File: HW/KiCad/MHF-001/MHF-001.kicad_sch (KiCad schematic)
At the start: 199 parts, among them J1 DE15_Socket_HighDensity_Mount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, J2 Mini-DIN-6, J3 Conn_Coaxial, J4 Conn_02x32_Odd_Even, J5 USB_B_Micro, J6 Conn_02x32_Odd_Even, J8 AVR-ISP-6, M3 CY7C109D-10ZXI, M5 CY7C109D-10ZXI, Q1 BC107, U1 ATMEGA2560-16AU, U10 74HC245, U11 74HC245, U12 74HC245, U13 CH340G, U14 AMS1117-5.0, U15 AMS1117-3.3, U2 74HC14, U3 74LS08, U4 74HC165, U6 74AHC373PW, U7 74HC595, U8 74HC595, U9 74HC157, Y1 16 MHz, Y2 12 MHz

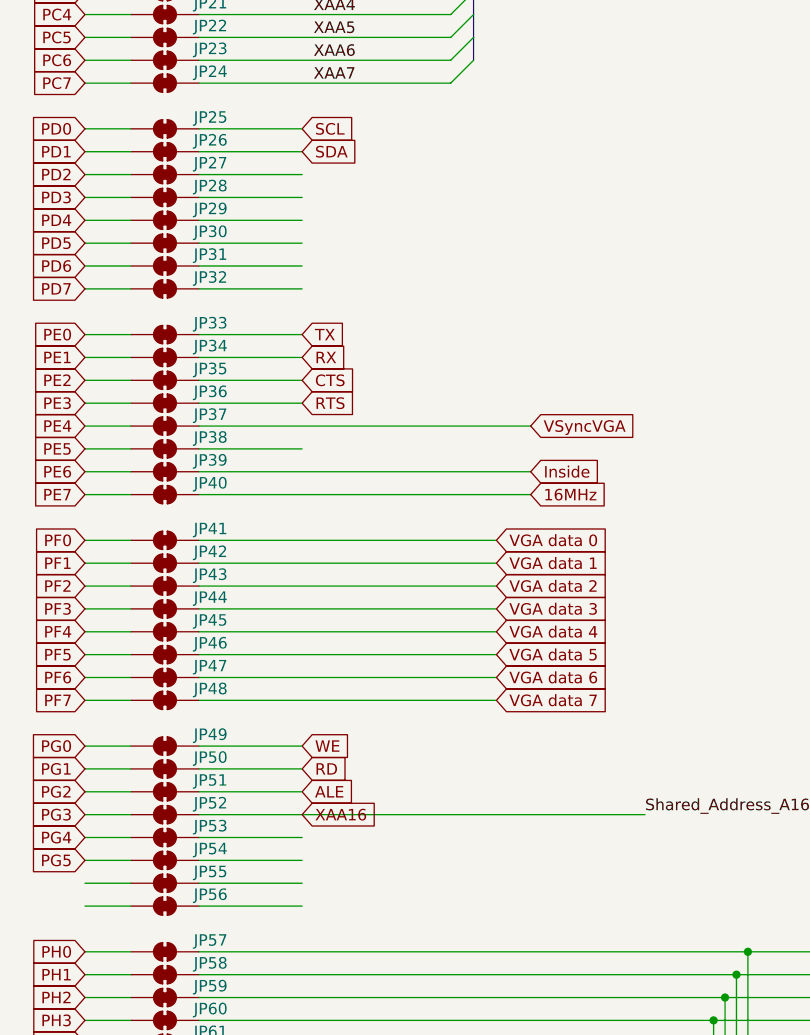
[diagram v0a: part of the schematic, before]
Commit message: some labels
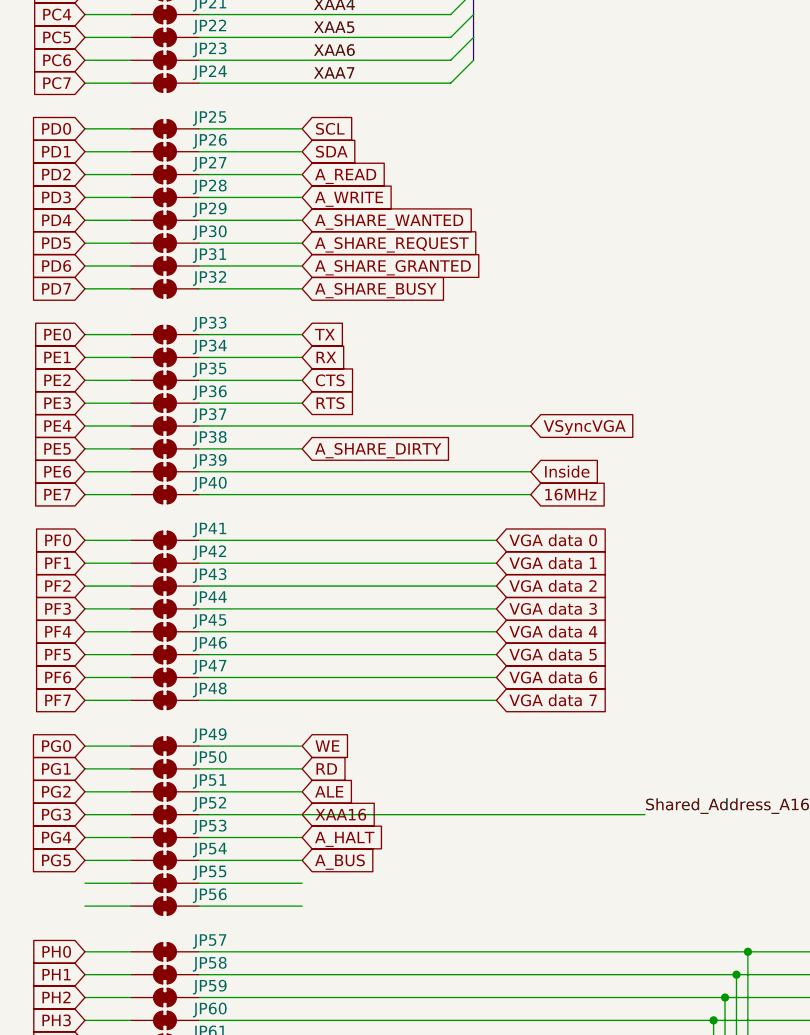
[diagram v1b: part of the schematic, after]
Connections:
- net A_BUS: now also JP54.2 (B)
- net A_HALT: now also JP53.2 (B)
- net A_READ: now also JP27.2 (B)
- net A_SHARE_BUSY: now also JP32.2 (B)
- net A_SHARE_DIRTY: now also JP38.2 (B)
- net A_SHARE_GRANTED: now also JP31.2 (B)
- net A_SHARE_REQUEST: now also JP30.2 (B)
- net A_SHARE_WANTED: now also JP29.2 (B)
- net A_WRITE: now also JP28.2 (B)
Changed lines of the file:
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@@
 		)
 	)
+	(global_label "A_SHARE_WANTED"
+		(shape input)
+		(at 675.64 426.72 0)
+		(fields_autoplaced yes)
+		(effects
+			(font
+				(size 1.27 1.27)
+			)
+			(justify left)
+		)
+		(property "Intersheetrefs" "${INTERSHEET_REFS}"
+			(at 694.9537 426.72 0)
+			(effects
+				(font
+					(size 1.27 1.27)
+				)
+				(justify left)
+				(hide yes)
+			)
+		)
+	)
 	(global_label "A[0..15]"
 		(shape input)
@@
 		)
 	)
+	(global_label "A_SHARE_REQUEST"
+		(shape input)
+		(at 675.64 429.26 0)
+		(fields_autoplaced yes)
+		(effects
+			(font
+				(size 1.27 1.27)
+			)
+			(justify left)
+		)
+		(property "Intersheetrefs" "${INTERSHEET_REFS}"
+			(at 696.1027 429.26 0)
+			(effects
+				(font
+					(size 1.27 1.27)
+				)
+				(justify left)
+				(hide yes)
+			)
+		)
+	)
 	(global_label "HSyncVGA"
 		(shape input)
@@
 		)
 	)
+	(global_label "A_SHARE_GRANTED"
+		(shape input)
+		(at 675.64 431.8 0)
+		(fields_autoplaced yes)
+		(effects
+			(font
+				(size 1.27 1.27)
+			)
+			(justify left)
+		)
+		(property "Intersheetrefs" "${INTERSHEET_REFS}"
+			(at 696.0423 431.8 0)
+			(effects
+				(font
+					(size 1.27 1.27)
+				)
+				(justify left)
+				(hide yes)
+			)
+		)
+	)
 	(global_label "PH1"
 		(shape input)
@@
 		)
 	)
+	(global_label "A_SHARE_DIRTY"
+		(shape input)
+		(at 675.64 452.12 0)
+		(fields_autoplaced yes)
+		(effects
+			(font
+				(size 1.27 1.27)
+			)
+			(justify left)
+		)
+		(property "Intersheetrefs" "${INTERSHEET_REFS}"
+			(at 692.8976 452.12 0)
+			(effects
+				(font
+					(size 1.27 1.27)
+				)
+				(justify left)
+				(hide yes)
+			)
+		)
+	)
 	(global_label "VGA data 5"
 		(shape input)
@@
 		)
 	)
+	(global_label "A_HALT"
+		(shape input)
+		(at 675.64 495.3 0)
+		(fields_autoplaced yes)
+		(effects
+			(font
+				(size 1.27 1.27)
+			)
+			(justify left)
+		)
+		(property "Intersheetrefs" "${INTERSHEET_REFS}"
+			(at 685.0962 495.3 0)
+			(effects
+				(font
+					(size 1.27 1.27)
+				)
+				(justify left)
+				(hide yes)
+			)
+		)
+	)
 	(global_label "Rf"
 		(shape input)
@@
 		)
 	)
+	(global_label "A_READ"
+		(shape input)
+		(at 675.64 421.64 0)
+		(fields_autoplaced yes)
+		(effects
+			(font
+				(size 1.27 1.27)
+			)
+			(justify left)
+		)
+		(property "Intersheetrefs" "${INTERSHEET_REFS}"
+			(at 685.459 421.64 0)
+			(effects
+				(font
+					(size 1.27 1.27)
+				)
+				(justify left)
+				(hide yes)
+			)
+		)
+	)
 	(global_label "A[0..15]"
 		(shape input)
@@
 		)
 	)
+	(global_label "A_SHARE_BUSY"
+		(shape input)
+		(at 675.64 434.34 0)
+		(fields_autoplaced yes)
+		(effects
+			(font
+				(size 1.27 1.27)
+			)
+			(justify left)
+		)
+		(property "Intersheetrefs" "${INTERSHEET_REFS}"
+			(at 692.5952 434.34 0)
+			(effects
+				(font
+					(size 1.27 1.27)
+				)
+				(justify left)
+				(hide yes)
+			)
+		)
+	)
 	(global_label "{RW,CLOCK,halt}"
 		(shape input)
@@
 		)
 	)
+	(global_label "A_WRITE"
+		(shape input)
+		(at 675.64 424.18 0)
+		(fields_autoplaced yes)
+		(effects
+			(font
+				(size 1.27 1.27)
+			)
+			(justify left)
+		)
+		(property "Intersheetrefs" "${INTERSHEET_REFS}"
+			(at 686.1242 424.18 0)
+			(effects
+				(font
+					(size 1.27 1.27)
+				)
+				(justify left)
+				(hide yes)
+			)
+		)
+	)
 	(global_label "SS"
 		(shape input)
@@
 				(hide yes)
 			)
+		)
+	)
+	(global_label "A_BUS"
+		(shape input)
+		(at 675.64 497.84 0)
+		(fields_autoplaced yes)
+		(effects
+			(font
+				(size 1.27 1.27)
+			)
+			(justify left)
+		)
+		(property "Intersheetrefs" "${INTERSHEET_REFS}"
+			(at 684.4914 497.84 0)
+			(effects
+				(font
+					(size 1.27 1.27)
+				)
+				(justify left)
+				(hide yes)
+			)

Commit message: schema MHF-001 maybe OK
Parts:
- removed sys_Addr1, sys_Addr2, sys_Data1: Conn_01x08, Connector_PinHeader_2.54mm:PinHeader_1x08_P2.54mm_Vertical, symbol Connector_Generic:Conn_01x08
- added J10: I2C, Connector_PinHeader_2.54mm:PinHeader_1x04_P2.54mm_Vertical, symbol Connector_Generic:Conn_01x04
- added J11: POWER, Connector_PinHeader_2.54mm:PinHeader_2x03_P2.54mm_Vertical, symbol Connector_Generic:Conn_02x03_Odd_Even
- added J7: SPI, Connector_PinHeader_2.54mm:PinHeader_1x06_P2.54mm_Vertical, symbol Connector_Generic:Conn_01x06
- added J9: Serial, Connector_PinHeader_2.54mm:PinHeader_1x06_P2.54mm_Vertical, symbol Connector_Generic:Conn_01x06
- added JP100, JP101, JP102, JP103, JP104, JP105, JP106, JP107, JP108, JP92, JP93, JP94, JP95, JP96, JP97, JP98, JP99: SolderJumper_3_Open, Jumper:SolderJumper-3_P1.3mm_Open_RoundedPad1.0x1.5mm, symbol Jumper:SolderJumper_3_Open
- added LED5, LED6: LED, LED_SMD:LED_0805_2012Metric, symbol Device:LED
- C10, C12, C13, C14, C15, C16, C2, C3, C4, C5, C6, C7, C8, C9: footprint Capacitor_SMD:C_0603_1608Metric -> Capacitor_SMD:C_0603_1608Metric_Pad1.08x0.95mm_HandSolder
- C11: footprint Capacitor_SMD:C_1206_3216Metric -> Capacitor_SMD:C_0603_1608Metric_Pad1.08x0.95mm_HandSolder
- J6: value Conn_02x32_Odd_Even -> 02x32
- LED1, LED2, LED3, LED4: footprint LED_SMD:LED_0201_0603Metric -> LED_SMD:LED_0805_2012Metric
- R24, R25, R26, R27, R28, R29, R30, R31, R32, R33, R34, R35, R36, R37: footprint Resistor_SMD:R_0603_1608Metric -> Resistor_SMD:R_0603_1608Metric_Pad0.98x0.95mm_HandSolder
- R38, R39: footprint (none) -> Resistor_SMD:R_0805_2012Metric_Pad1.20x1.40mm_HandSolder
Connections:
- net ~{MidRAM} is gone; now on net GND: M5.30 (~{CS1}/~{CE1})
- net ~{Read} is gone; now on net S_READ: M5.32 (~{OE})
- net ~{SUPRESS} is gone; now on net VGA data 3: U3.2
- net ~{Write} is gone; now on net S_WRITE: M5.5 (~{WE})
- net +5V: now also J4.1 (Pin_1), J4.2 (Pin_2), J6.1 (Pin_1), J6.2 (Pin_2), J10.4 (Pin_4), J7.6 (Pin_6), J9.6 (Pin_6)
- net A0: now also J4.11 (Pin_11), J6.11 (Pin_11)
- net A1: now also J4.12 (Pin_12), J6.12 (Pin_12)
- net A10: now also J4.21 (Pin_21), J6.21 (Pin_21)
- net A11: now also J4.22 (Pin_22), J6.22 (Pin_22)
- net A12: now also J4.23 (Pin_23), J6.23 (Pin_23)
- net A13: now also J4.24 (Pin_24), J6.24 (Pin_24)
- net A14: now also J4.25 (Pin_25), J6.25 (Pin_25)
- net A15: now also J4.26 (Pin_26), J6.26 (Pin_26)
- net A2: now also J4.13 (Pin_13), J6.13 (Pin_13)
- net A3: now also J4.14 (Pin_14), J6.14 (Pin_14)
- net A4: now also J4.15 (Pin_15), J6.15 (Pin_15)
- net A5: now also J4.16 (Pin_16), J6.16 (Pin_16)
- net A6: now also J4.17 (Pin_17), J6.17 (Pin_17)
- net A7: now also J4.18 (Pin_18), J6.18 (Pin_18)
- net A8: now also J4.19 (Pin_19), J6.19 (Pin_19)
- net A9: now also J4.20 (Pin_20), J6.20 (Pin_20)
- net A_BUS: now also J4.29 (Pin_29), J6.29 (Pin_29), JP93.1 (A); no longer JP54.2 (B)
- net A_HALT: now also J4.31 (Pin_31), J6.31 (Pin_31), JP94.1 (A); no longer JP53.2 (B)
- net A_READ: now also J4.33 (Pin_33), J6.33 (Pin_33), JP95.1 (A); no longer JP27.2 (B)
- net A_SHARE_BUSY: now also J4.37 (Pin_37), J6.37 (Pin_37), JP97.1 (A); no longer JP32.2 (B)
- net A_SHARE_DIRTY: now also J4.39 (Pin_39), J6.39 (Pin_39), JP98.1 (A); no longer JP38.2 (B)
- net A_SHARE_GRANTED: now also J4.41 (Pin_41), J6.41 (Pin_41), JP99.1 (A); no longer JP31.2 (B)
- net A_SHARE_REQUEST: now also J4.43 (Pin_43), J6.43 (Pin_43), JP100.1 (A); no longer JP30.2 (B)
- net A_SHARE_WANTED: now also J4.45 (Pin_45), J6.45 (Pin_45), JP101.1 (A); no longer JP29.2 (B)
- net A_WRITE: now also J4.35 (Pin_35), J6.35 (Pin_35), JP96.1 (A); no longer JP28.2 (B)
- net CTS: now also R38.2, J9.2 (Pin_2)
- net D0: now also J4.3 (Pin_3), J6.3 (Pin_3); no longer J4.1 (Pin_1), J6.1 (Pin_1)
- net D1: now also J4.4 (Pin_4), J6.4 (Pin_4); no longer J4.2 (Pin_2), J6.2 (Pin_2)
- net D2: now also J4.5 (Pin_5), J6.5 (Pin_5); no longer J4.3 (Pin_3), J6.3 (Pin_3)
- net D3: now also J4.6 (Pin_6), J6.6 (Pin_6); no longer J4.4 (Pin_4), J6.4 (Pin_4)
- net D4: now also J4.7 (Pin_7), J6.7 (Pin_7); no longer J4.5 (Pin_5), J6.5 (Pin_5)
- net D5: now also J4.8 (Pin_8), J6.8 (Pin_8)
- net D6: now also J4.9 (Pin_9), J6.9 (Pin_9); no longer J4.7 (Pin_7), J6.7 (Pin_7)
- net D7: now also J4.10 (Pin_10), J6.10 (Pin_10)
- net GND: now also J4.63 (Pin_63), J4.64 (Pin_64), J5.6 (Shield), J6.63 (Pin_63), J6.64 (Pin_64), J10.3 (Pin_3), J11.2 (Pin_2), J11.4 (Pin_4), J11.6 (Pin_6), J7.5 (Pin_5), J9.5 (Pin_5), LED5.1 (K), LED6.1 (K)
- net G_A_DIR: now also U11.1 (A->B), U12.1 (A->B), JP107.2 (C)
- net G_A_OE: now also U11.19 (CE), U12.19 (CE), JP108.2 (C)
- net G_D_DIR: now also U10.1 (A->B), JP105.2 (C)
- net G_D_OE: now also U10.19 (CE), JP106.2 (C)
- net MISO: now also J7.1 (Pin_1)
- net MOSI: now also JP56.1 (A), J7.2 (Pin_2)
- net Mega_6309_data0: now also JP41.2 (B); no longer JP81.2 (B)
- net Mega_6309_data1: now also JP42.2 (B); no longer JP82.2 (B)
- net Mega_6309_data2: now also JP43.2 (B); no longer JP83.2 (B)
- net Mega_6309_data3: now also JP44.2 (B); no longer JP84.2 (B)
- net Mega_6309_data4: now also JP45.2 (B); no longer JP85.2 (B)
- net Mega_6309_data5: now also JP46.2 (B); no longer JP86.2 (B)
- net Mega_6309_data6: now also JP47.2 (B); no longer JP87.2 (B)
- net Mega_6309_data7: now also JP48.2 (B); no longer JP88.2 (B)
- net PS2 Clock: now also JP56.2 (B)
- net PS2 Data: now also JP55.2 (B)
- net RTS: now also R39.2, J9.1 (Pin_1)
- net RX: now also J9.3 (Pin_3)
- net SCK: now also JP55.1 (A), J7.3 (Pin_3)
- net SCL: now also J10.2 (Pin_2)
- net SDA: now also J10.1 (Pin_1)
- net SS: now also J7.4 (Pin_4)
- net SYNC_RCA: now also JP85.2 (B), U4.3 (D4)
- net S_READ: now also JP103.2 (C)
- net S_WRITE: now also JP104.2 (C)
- net TX: now also J9.4 (Pin_4)
- net VGA data 0: now also JP81.2 (B); no longer JP41.2 (B)
- net VGA data 1: now also JP82.2 (B); no longer JP42.2 (B)
- net VGA data 2: now also JP83.2 (B); no longer JP43.2 (B)
- net VGA data 3: now also JP84.2 (B); no longer JP44.2 (B)
- net VGA data 5: now also JP86.2 (B); no longer JP46.2 (B)
- net VGA data 6: now also JP87.2 (B); no longer JP47.2 (B)
- net VGA data 7: now also JP88.2 (B); no longer JP48.2 (B)
- net VIN: now also J11.1 (Pin_1), J11.3 (Pin_3), J11.5 (Pin_5)
- net XAA16: no longer M5.10 (A16)
- net Shared_Address_A16: now reaches JP14.2 (B)
- net Shared_Address_A16: now also M5.10 (A16), JP92.2 (C)
- net A16: now reaches J6.27 (Pin_27)
- net A16: now also J4.27 (Pin_27), JP92.1 (A)
- net B16: now reaches J6.28 (Pin_28)
- net B16: now also J4.28 (Pin_28), JP92.3 (B)
- net B_BUS: now reaches J6.30 (Pin_30)
- net B_BUS: now also J4.30 (Pin_30), JP93.3 (B)
- net B_HALT: now reaches J6.32 (Pin_32)
- net B_HALT: now also J4.32 (Pin_32), JP94.3 (B)
- net B_READ: now reaches J6.34 (Pin_34)
- net B_READ: now also J4.34 (Pin_34), JP95.3 (B)
- net B_WRITE: now reaches J6.36 (Pin_36)
- net B_WRITE: now also J4.36 (Pin_36), JP96.3 (B)
- net B_SHARE_BUSY: now reaches J6.38 (Pin_38)
- net B_SHARE_BUSY: now also J4.38 (Pin_38), JP97.3 (B)
- net B_SHARE_DIRTY: now reaches J6.40 (Pin_40)
- net B_SHARE_DIRTY: now also J4.40 (Pin_40), JP98.3 (B)
- net B_SHARE_GRANTED: now reaches J6.42 (Pin_42)
- net B_SHARE_GRANTED: now also J4.42 (Pin_42), JP99.3 (B)
- net B_SHARE_REQUEST: now reaches J6.44 (Pin_44)
- net B_SHARE_REQUEST: now also J4.44 (Pin_44), JP100.3 (B)
- net B_SHARE_WANTED: now reaches J6.46 (Pin_46)
- net B_SHARE_WANTED: now also J4.46 (Pin_46), JP101.3 (B)
- net A_S_ENABLE: now reaches J6.47 (Pin_47)
- net A_S_ENABLE: now also J4.47 (Pin_47), JP102.1 (A)
- net B_S_ENABLE: now reaches J6.48 (Pin_48)
- net B_S_ENABLE: now also J4.48 (Pin_48), JP102.3 (B)
- net A_S_READ: now reaches J6.49 (Pin_49)
- net A_S_READ: now also J4.49 (Pin_49), JP103.1 (A)
- net B_S_READ: now reaches J6.50 (Pin_50)
- net B_S_READ: now also J4.50 (Pin_50), JP103.3 (B)
- net A_S_WRITE: now reaches J6.51 (Pin_51)
- net A_S_WRITE: now also J4.51 (Pin_51), JP104.1 (A)
- net B_S_WRITE: now reaches J6.52 (Pin_52)
- net B_S_WRITE: now also J4.52 (Pin_52), JP104.3 (B)
- net A_G_D_DIR: now reaches J6.53 (Pin_53)
- net A_G_D_DIR: now also J4.53 (Pin_53), JP105.1 (A)
- net B_G_D_DIR: now reaches J6.54 (Pin_54)
- net B_G_D_DIR: now also J4.54 (Pin_54), JP105.3 (B)
- net A_G_D_OE: now reaches J6.55 (Pin_55)
- net A_G_D_OE: now also J4.55 (Pin_55), JP106.1 (A)
- net B_G_D_OE: now reaches J6.56 (Pin_56)
- net B_G_D_OE: now also J4.56 (Pin_56), JP106.3 (B)
- net A_G_A_DIR: now reaches J6.57 (Pin_57)
- net A_G_A_DIR: now also J4.57 (Pin_57), JP107.1 (A)
- net B_G_A_DIR: now reaches J6.58 (Pin_58)
- net B_G_A_DIR: now also J4.58 (Pin_58), JP107.3 (B)
- net A_G_A_OE: now reaches J6.59 (Pin_59)
- net A_G_A_OE: now also J4.59 (Pin_59), JP108.1 (A)
- net B_G_A_OE: now reaches J6.60 (Pin_60)
- net B_G_A_OE: now also J4.60 (Pin_60), JP108.3 (B)
- net PS2-OE: now reaches U7.13 (~{OE}), U8.13 (~{OE})
- net PS2-OE: now also JP13.2 (B)
- net S_ENABLE: now reaches M5.6 (CS2/CE2)
- net S_ENABLE: now also JP102.2 (C)
- net at R38.1: now also LED5.2 (A)
- net at R39.1: now also LED6.2 (A)
- removed net VGA data 4: JP45.2 (B), U4.3 (D4)
- new net X_BUS: JP54.2 (B), JP93.2 (C)
- new net X_HALT: JP53.2 (B), JP94.2 (C)
- new net X_READ: JP27.2 (B), JP95.2 (C)
- new net X_SHARE_BUSY: JP29.2 (B), JP97.2 (C)
- new net X_SHARE_DIRTY: JP30.2 (B), JP98.2 (C)
- new net X_SHARE_GRANTED: JP31.2 (B), JP99.2 (C)
- new net X_SHARE_REQUEST: JP100.2 (C), JP32.2 (B)
- new net X_SHARE_WANTED: JP101.2 (C), JP38.2 (B)
- new net X_WRITE: JP28.2 (B), JP96.2 (C)
- no-connect marks 25 -> 26
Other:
- note removed: "ATF1504"
- note removed: "Arduino"
- note removed: "HD6309"
- note removed: "RAM-shared"
- note removed: "RAM-system"
- note removed: "gate-address"
- note removed: "gate-data"
- moved on the sheet: H5, H6, H7, H8, J1, J4, J6, JP55, JP56, R14, R15
